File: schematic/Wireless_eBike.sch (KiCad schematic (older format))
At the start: 7 parts

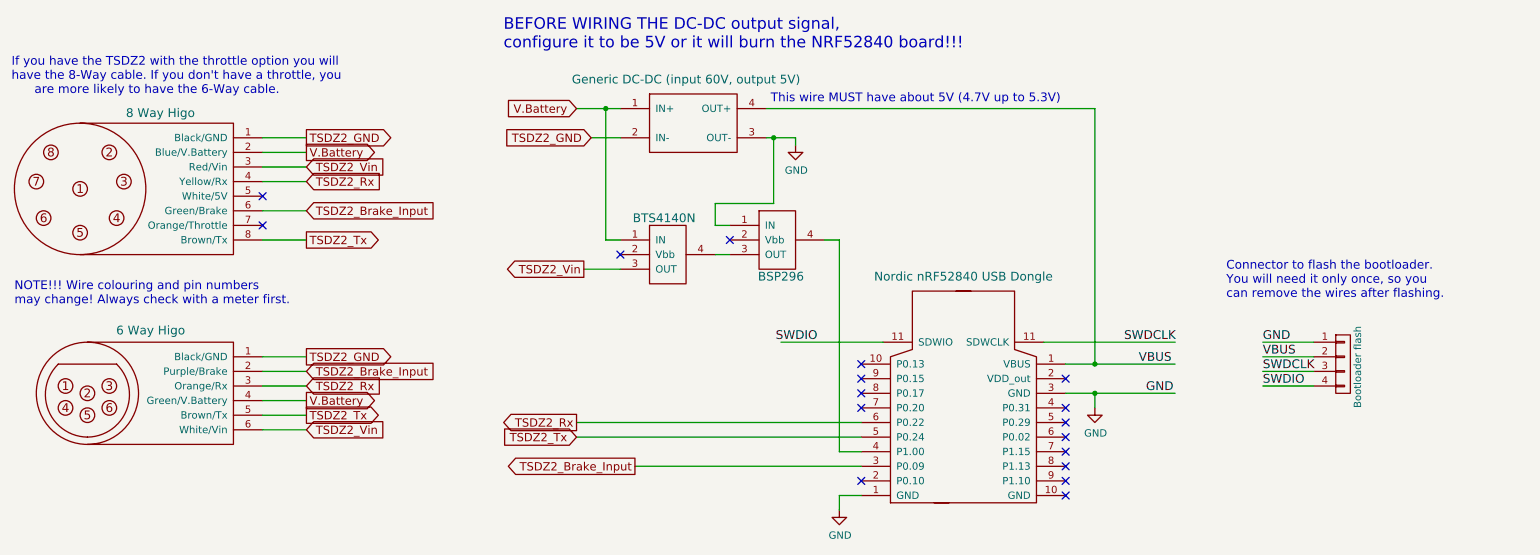
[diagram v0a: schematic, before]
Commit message: updated schematic
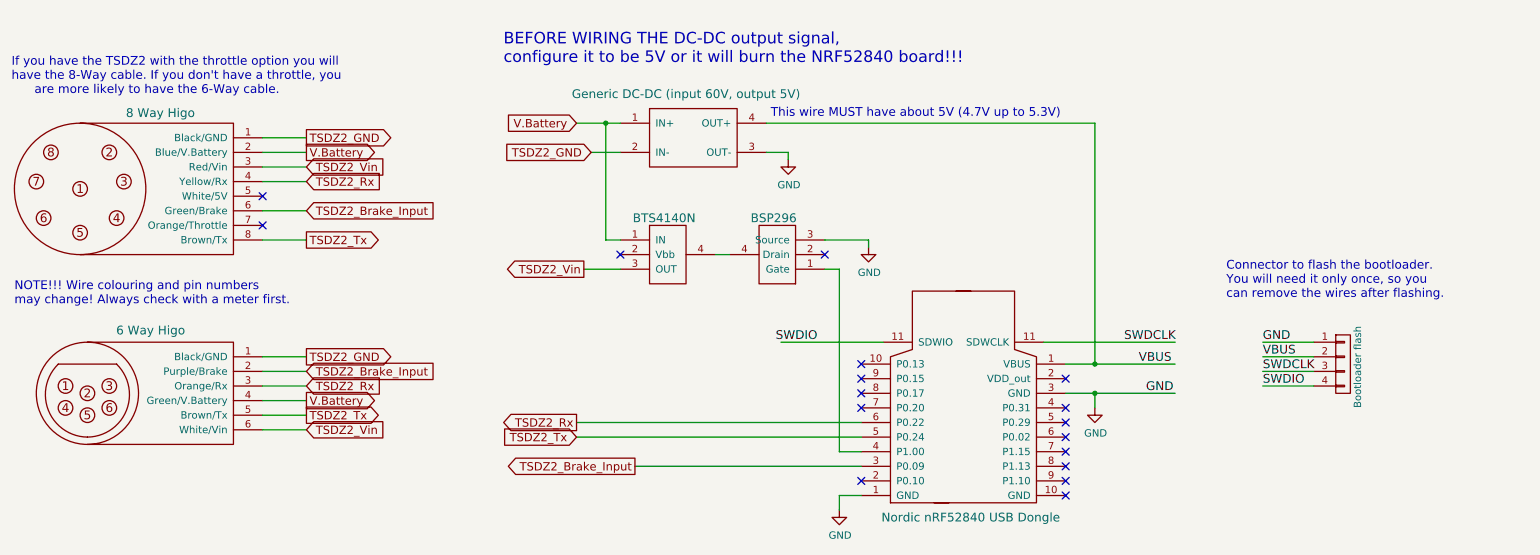
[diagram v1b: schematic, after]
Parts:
- removed U?: BSP296, symbol Wireless_eBike:BTS4140N-Wireless_eBike
- added U?: BSP296, symbol Wireless_eBike:BSP296
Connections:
- wire segments 47 -> 44
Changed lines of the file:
@@
 Text GLabel 2850 4200 2    57   Input ~ 0
 TSDZ2_Rx
-Text GLabel 4700 2300 0    57   Input ~ 0
+Text GLabel 4700 2400 0    57   Input ~ 0
 V.Battery
 Text GLabel 4700 4450 0    57   Output ~ 0
@@
 Text GLabel 4700 4550 0    57   Input ~ 0
 TSDZ2_Tx
-Text Notes 4200 1900 0    79   ~ 0
+Text Notes 4200 2000 0    79   ~ 0
 BEFORE WIRING THE DC-DC output signal,\nconfigure it to be 5V or it will burn the NRF52840 board!!!
 Text GLabel 2850 4000 2    57   Output ~ 0
@@
 Text GLabel 2850 2500 2    57   Output ~ 0
 TSDZ2_GND
-Text GLabel 4800 2500 0    57   Input ~ 0
+Text GLabel 4800 2600 0    57   Input ~ 0
 TSDZ2_GND
 Wire Wire Line
@@
 	2850 4500 2550 4500
 Wire Wire Line
-	4800 2500 5000 2500
+	4800 2600 5000 2600
 Text Notes 830  2210 0    60   ~ 0
 If you have the TSDZ2 with the throttle option you will\nhave the 8-Way cable. If you don't have a throttle, you\n      are more likely to have the 6-Way cable.
@@
 P 7350 4400
 F 0 "U?" H 7350 4400 60  0001 C CNN
-F 1 "Nordic nRF52840 USB Dongle" H 7350 5350 60  0000 C CNN
+F 1 "Nordic nRF52840 USB Dongle" H 7400 3700 60  0000 C CNN
 F 2 "" H 7200 4250 60  0000 C CNN
 F 3 "" H 7200 4250 60  0000 C CNN
@@
 	8250 4050 8050 4050
 Wire Wire Line
-	4700 2300 4900 2300
-Wire Wire Line
-	5650 3300 5750 3300
+	4700 2400 4900 2400
 Wire Wire Line
 	6650 4450 4700 4450
@@
 L power:GND #PWR?
 U 1 1 6013E89A
-P 6200 2550
-F 0 "#PWR?" H 6200 2300 50  0001 C CNN
-F 1 "GND" H 6205 2377 50  0000 C CNN
-F 2 "" H 6200 2550 50  0001 C CNN
-F 3 "" H 6200 2550 50  0001 C CNN
-	1    6200 2550
-	1    0    0    -1
-$EndComp
-Wire Wire Line
-	6200 2500 6200 2550
-Wire Wire Line
-	6000 2500 6050 2500
-Wire Wire Line
-	5750 3100 5650 3100
-Wire Wire Line
-	5650 3100 5650 2950
-Wire Wire Line
-	5650 2950 6050 2950
-Wire Wire Line
-	6050 2950 6050 2500
-Connection ~ 6050 2500
-Wire Wire Line
-	6050 2500 6200 2500
-Wire Wire Line
-	6500 3200 6500 4650
-Wire Wire Line
-	6400 3200 6500 3200
-Wire Wire Line
-	8250 2300 8250 4050
-Wire Wire Line
-	6000 2300 8250 2300
+P 6150 2650
+F 0 "#PWR?" H 6150 2400 50  0001 C CNN
+F 1 "GND" H 6155 2477 50  0000 C CNN
+F 2 "" H 6150 2650 50  0001 C CNN
+F 3 "" H 6150 2650 50  0001 C CNN
+	1    6150 2650
+	1    0    0    -1
+$EndComp
+Wire Wire Line
+	8250 2400 8250 4050
+Wire Wire Line
+	6000 2400 8250 2400
 Text GLabel 5100 4750 0    57   Output ~ 0
 TSDZ2_Brake_Input
@@
 	5000 3200 4900 3200
 Wire Wire Line
-	4900 3200 4900 2300
-Connection ~ 4900 2300
-Wire Wire Line
-	4900 2300 5000 2300
+	4900 3200 4900 2400
+Connection ~ 4900 2400
+Wire Wire Line
+	4900 2400 5000 2400
 Text Label 9400 3900 0    60   ~ 0
 GND
@@
 NoConn ~ 8050 4850
 NoConn ~ 8050 4950
-NoConn ~ 5750 3200
 NoConn ~ 5000 3300
 Text Notes 9150 3800 0    60   ~ 0
 Connector to flash the bootloader.\nYou will need it only once, so you\ncan remove the wires after flashing.\n\n\n
-Text Notes 6030 2460 0    60   ~ 0
+Text Notes 6030 2560 0    60   ~ 0
 This wire MUST have about 5V (4.7V up to 5.3V)\n\n\n
 Text Label 8450 3900 0    60   ~ 0
@@
 L Wireless_eBike:Generic_DC-DC-Wireless_eBike U?
 U 1 1 60103A2E
-P 5500 2400
-F 0 "U?" H 5500 2787 60  0001 C CNN
-F 1 "Generic DC-DC (input 60V, output 5V)" H 5450 2700 60  0000 C CNN
-F 2 "" H 5450 2400 60  0000 C CNN
-F 3 "" H 5450 2400 60  0000 C CNN
-	1    5500 2400
-	1    0    0    -1
-$EndComp
+P 5500 2500
+F 0 "U?" H 5500 2887 60  0001 C CNN
+F 1 "Generic DC-DC (input 60V, output 5V)" H 5450 2800 60  0000 C CNN
+F 2 "" H 5450 2500 60  0000 C CNN
+F 3 "" H 5450 2500 60  0000 C CNN
+	1    5500 2500
+	1    0    0    -1
+$EndComp
+$Comp
+L Wireless_eBike:CONN_01X04-Wireless_eBike P?
+U 1 1 60034D62
+P 9950 4050
+F 0 "P?" H 10028 4091 50  0001 L CNN
+F 1 "Bootloader flash" V 10050 3750 50  0000 L CNN
+F 2 "" H 9950 4050 50  0000 C CNN
+F 3 "" H 9950 4050 50  0000 C CNN
+	1    9950 4050
+	1    0    0    -1
+$EndComp
+Wire Wire Line
+	6500 3400 6500 4650
+NoConn ~ 6400 3300
+Wire Wire Line
+	5750 3300 5650 3300
+Wire Wire Line
+	6400 3400 6500 3400
+Wire Wire Line
+	6150 2600 6150 2650
 $Comp
 L Wireless_eBike:BTS4140N-Wireless_eBike U?
@@
 	1    0    0    -1
 $EndComp
-$Comp
-L Wireless_eBike:BTS4140N-Wireless_eBike U?
-U 1 1 60105AA1
-P 6100 3200
-F 0 "U?" H 6075 3587 60  0001 C CNN
-F 1 "BSP296" H 6100 2950 60  0000 C CNN
-F 2 "" H 5500 3250 60  0000 C CNN
-F 3 "" H 5500 3250 60  0000 C CNN
-	1    6100 3200
-	1    0    0    -1
-$EndComp
-$Comp
-L Wireless_eBike:CONN_01X04-Wireless_eBike P?
-U 1 1 60034D62
-P 9950 4050
-F 0 "P?" H 10028 4091 50  0001 L CNN
-F 1 "Bootloader flash" V 10050 3750 50  0000 L CNN
-F 2 "" H 9950 4050 50  0000 C CNN
-F 3 "" H 9950 4050 50  0000 C CNN
-	1    9950 4050
-	1    0    0    -1
+Wire Wire Line
+	6000 2600 6150 2600
+$Comp
+L power:GND #PWR?
+U 1 1 6005D0CE
+P 6700 3250
+F 0 "#PWR?" H 6700 3000 50  0001 C CNN
+F 1 "GND" H 6705 3077 50  0000 C CNN
+F 2 "" H 6700 3250 50  0001 C CNN
+F 3 "" H 6700 3250 50  0001 C CNN
+	1    6700 3250
+	1    0    0    -1
+$EndComp
+Wire Wire Line
+	6700 3200 6700 3250
+Wire Wire Line
+	6400 3200 6700 3200
+$Comp
+L Wireless_eBike:BSP296 U?
+U 1 1 6006EF16
+P 6050 3300
+F 0 "U?" H 6025 2913 60  0001 C CNN
+F 1 "BSP296" H 6050 3050 60  0000 C CNN
+F 2 "" H 5450 3350 60  0000 C CNN
+F 3 "" H 5450 3350 60  0000 C CNN
+	1    6050 3300
+	-1   0    0    1
 $EndComp
 $EndSCHEMATC
